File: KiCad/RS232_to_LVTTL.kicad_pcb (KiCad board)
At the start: 2 copper layers, 36.1 x 34 mm, 22 parts, among them J1 DB25_Female, J2 Conn_01x05, U1 TPS54308, U2 MAX3232

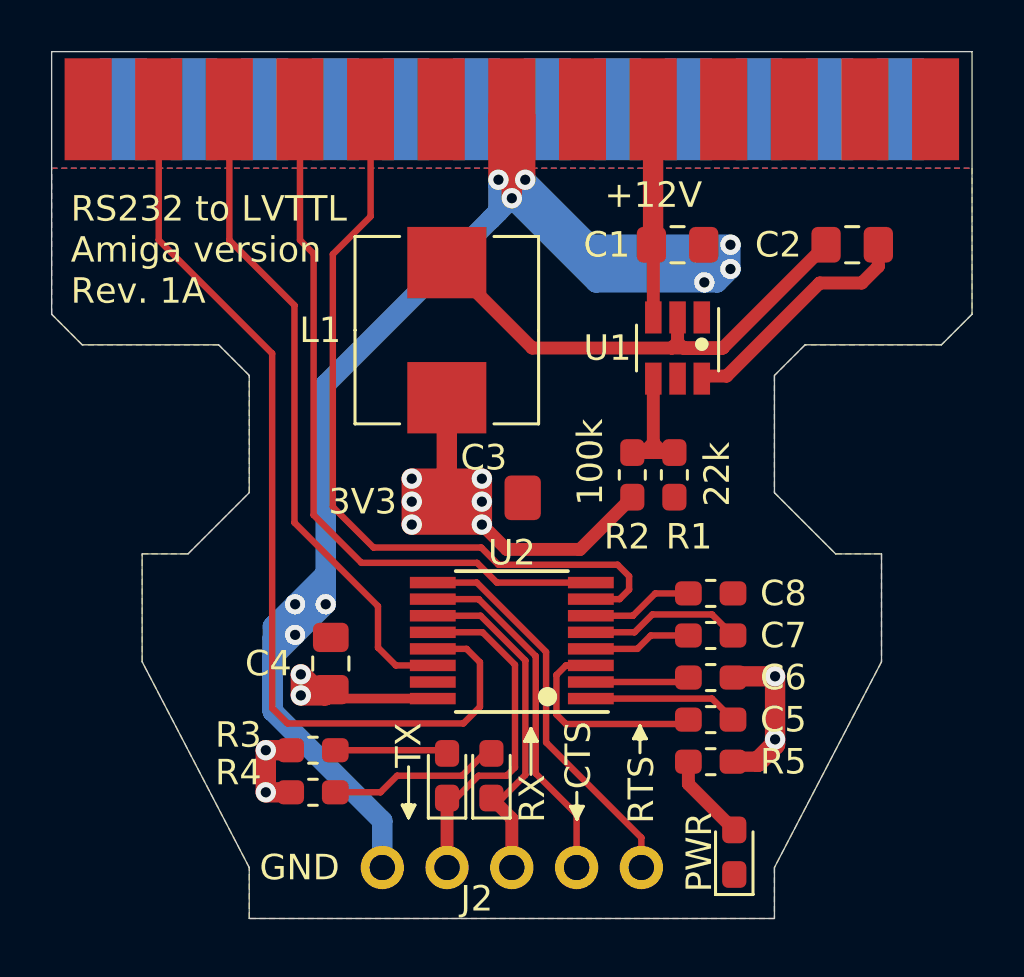
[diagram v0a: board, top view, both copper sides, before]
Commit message: some small routing and silkscreen fixes
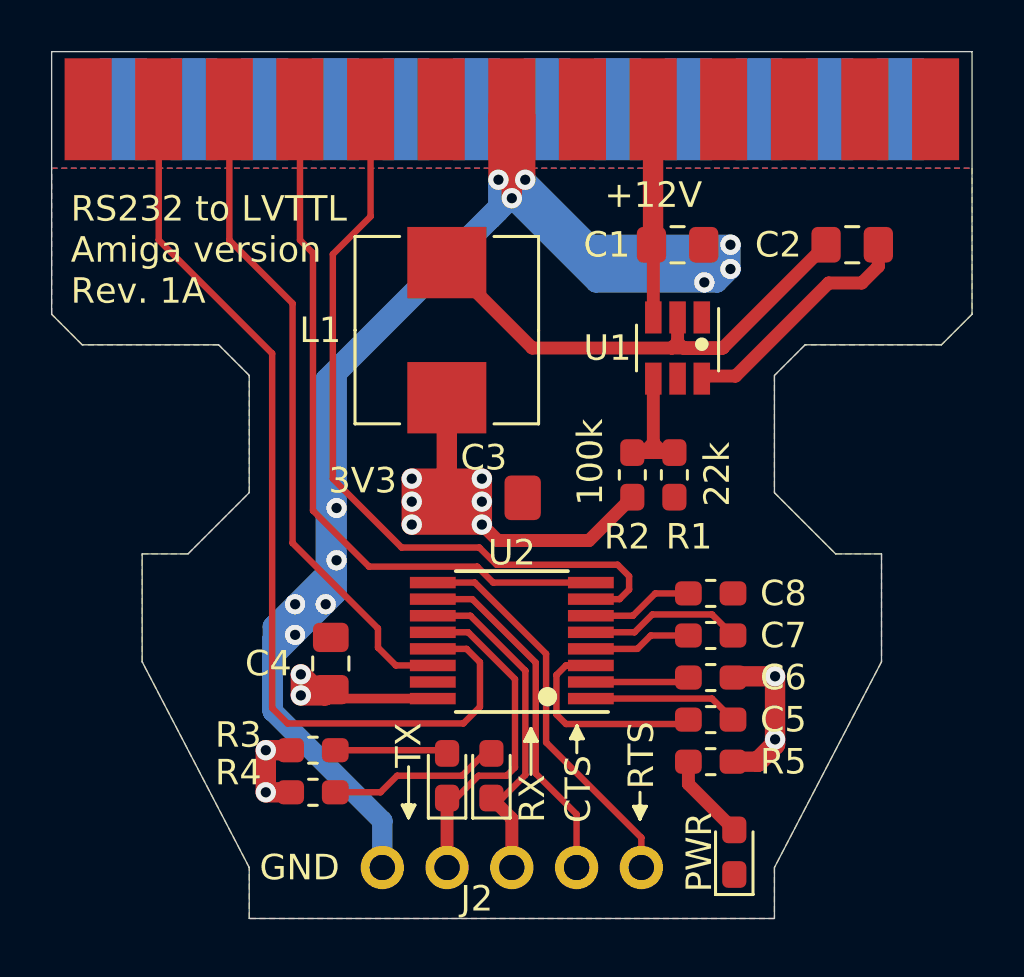
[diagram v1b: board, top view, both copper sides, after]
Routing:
- net GND: track 91.4 -> 113.5 mm, vias 9 -> 11
- net CTS: track 31.5 -> 30.9 mm
